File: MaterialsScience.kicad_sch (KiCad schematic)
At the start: 1 part, among them U1 LM555xN

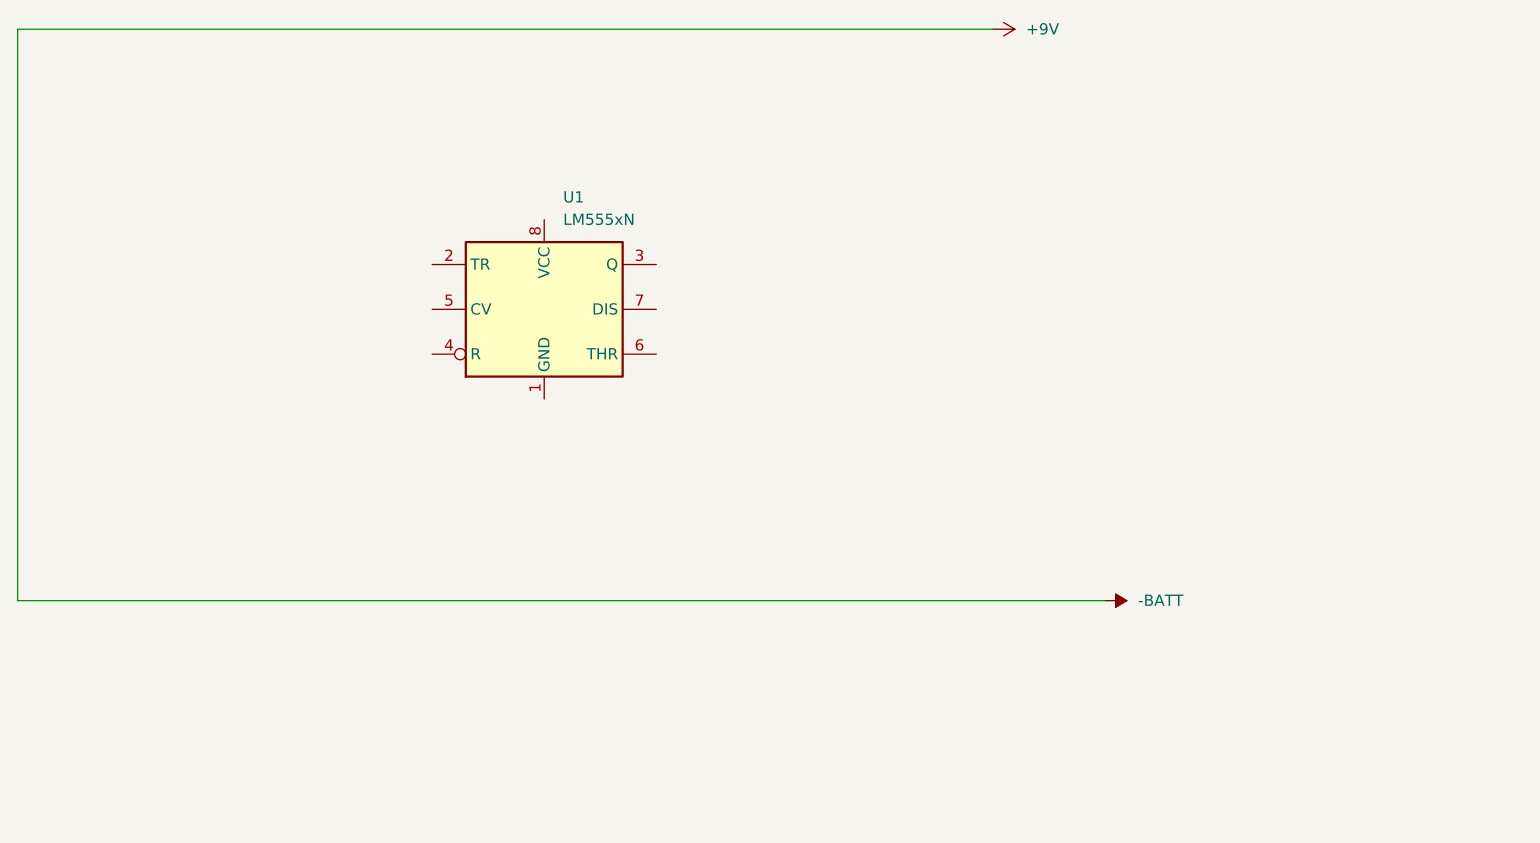
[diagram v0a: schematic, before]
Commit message: Add files via upload
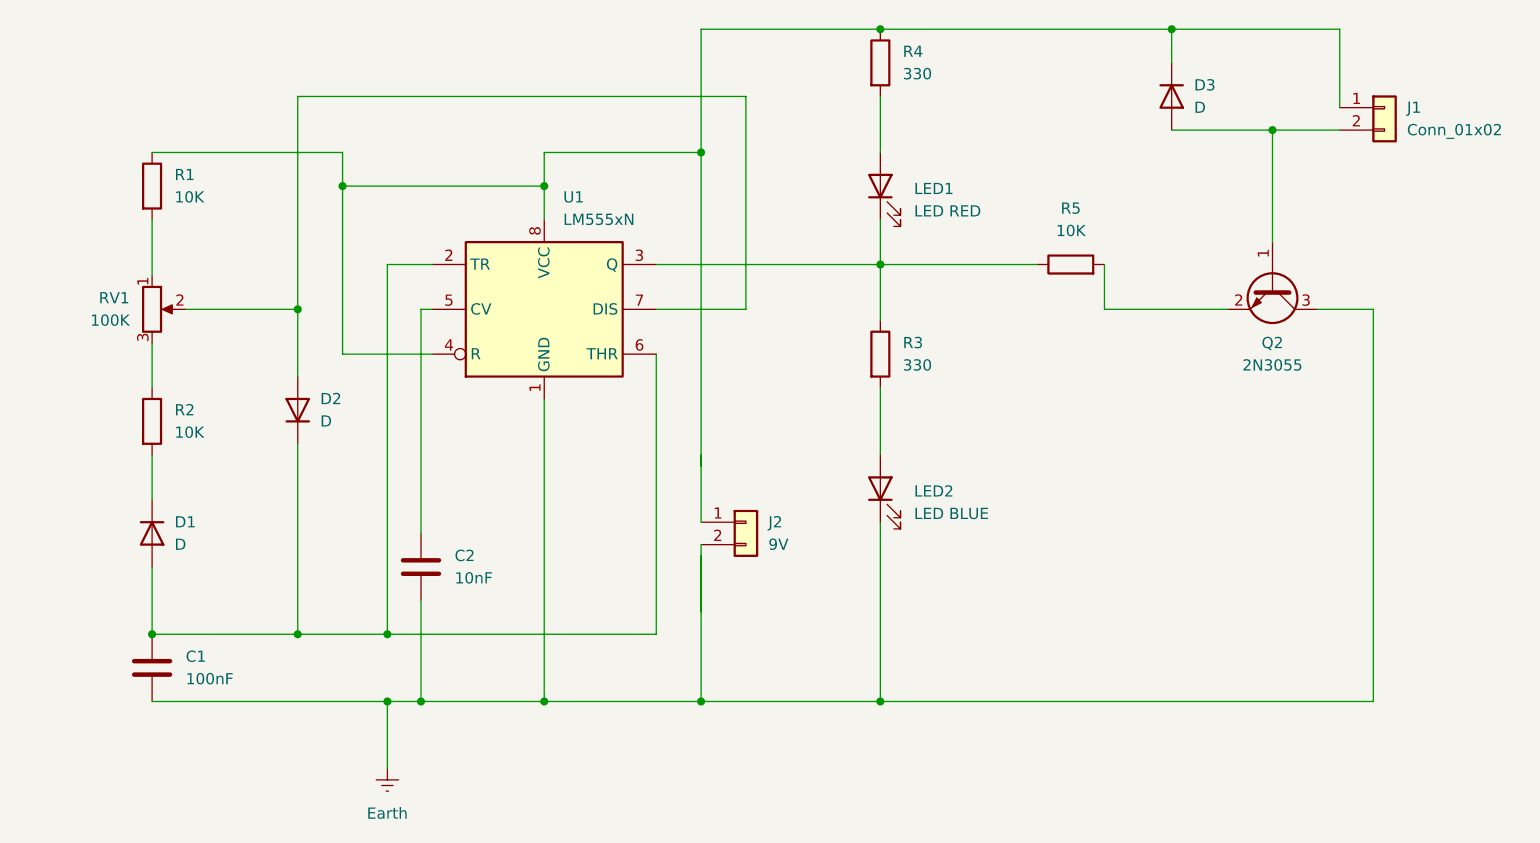
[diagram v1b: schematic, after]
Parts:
- added C1: 100nF, Capacitor_THT:C_Disc_D5.0mm_W2.5mm_P2.50mm, symbol Device:C
- added C2: 10nF, Capacitor_THT:C_Disc_D5.0mm_W2.5mm_P2.50mm, symbol Device:C
- added D1, D2, D3: D, Diode_THT:D_DO-41_SOD81_P10.16mm_Horizontal, symbol Device:D
- added J1: Conn_01x02, Connector_PinHeader_2.54mm:PinHeader_1x02_P2.54mm_Vertical, symbol Connector_Generic:Conn_01x02
- added J2: 9V, Connector_PinHeader_2.54mm:PinHeader_1x02_P2.54mm_Vertical, symbol Connector_Generic:Conn_01x02
- added LED1: LED RED, LED_THT:LED_D5.0mm, symbol Device:LED
- added LED2: LED BLUE, LED_THT:LED_D5.0mm, symbol Device:LED
- added Q2: 2N3055, Package_TO_SOT_THT:TO-3, symbol Transistor_BJT:2N3055
- added R1, R2, R5: 10K, Resistor_THT:R_Axial_DIN0207_L6.3mm_D2.5mm_P7.62mm_Horizontal, symbol Device:R
- added R3, R4: 330, Resistor_THT:R_Axial_DIN0207_L6.3mm_D2.5mm_P7.62mm_Horizontal, symbol Device:R
- added RV1: 100K, Potentiometer_THT:Potentiometer_Bourns_3296W_Vertical, symbol Device:R_Potentiometer
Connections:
- net Earth: now reaches U1.1 (GND)
- net Earth: now also C1.2, C2.2, J2.2 (Pin_2), LED2.1 (K), Q2.3 (C)
- net at U1.2 (TR): now also U1.6 (THR), C1.1, D1.2 (A), D2.1 (K)
- net at U1.3 (Q): now also LED1.1 (K), R3.1, R5.1
- net at U1.4 (R): now also U1.8 (VCC), D3.1 (K), J1.1 (Pin_1), J2.1 (Pin_1), R1.1, R4.1
- net at U1.5 (CV): now also C2.1
- net at U1.7 (DIS): now also D2.2 (A), RV1.2
- new net: R1.2, RV1.1
- new net: Q2.2 (E), R5.2
- new net: R2.1, RV1.3
- new net: D1.1 (K), R2.2
- new net: D3.2 (A), J1.2 (Pin_2), Q2.1 (B)
- new net: LED1.2 (A), R4.2
- new net: LED2.2 (A), R3.2
